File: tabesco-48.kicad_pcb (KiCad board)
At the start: 2 copper layers, 196.2 x 86.7 mm, 64 parts, among them U1 ProMicro

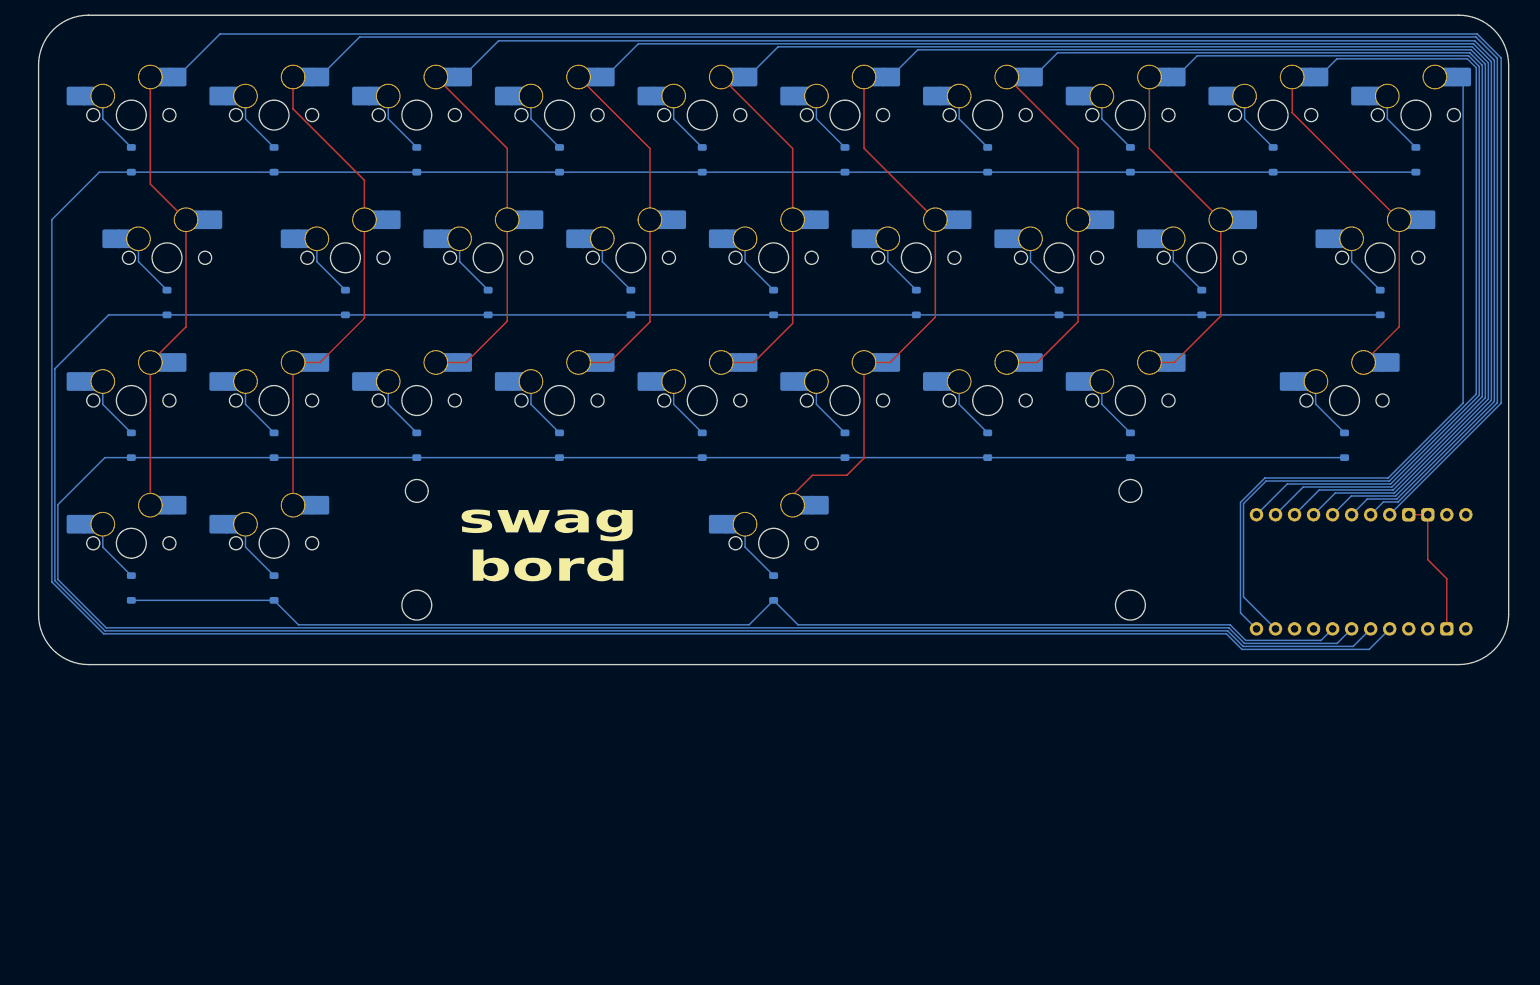
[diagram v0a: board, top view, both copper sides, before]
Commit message: more work, transitioning to IC in seperate repo
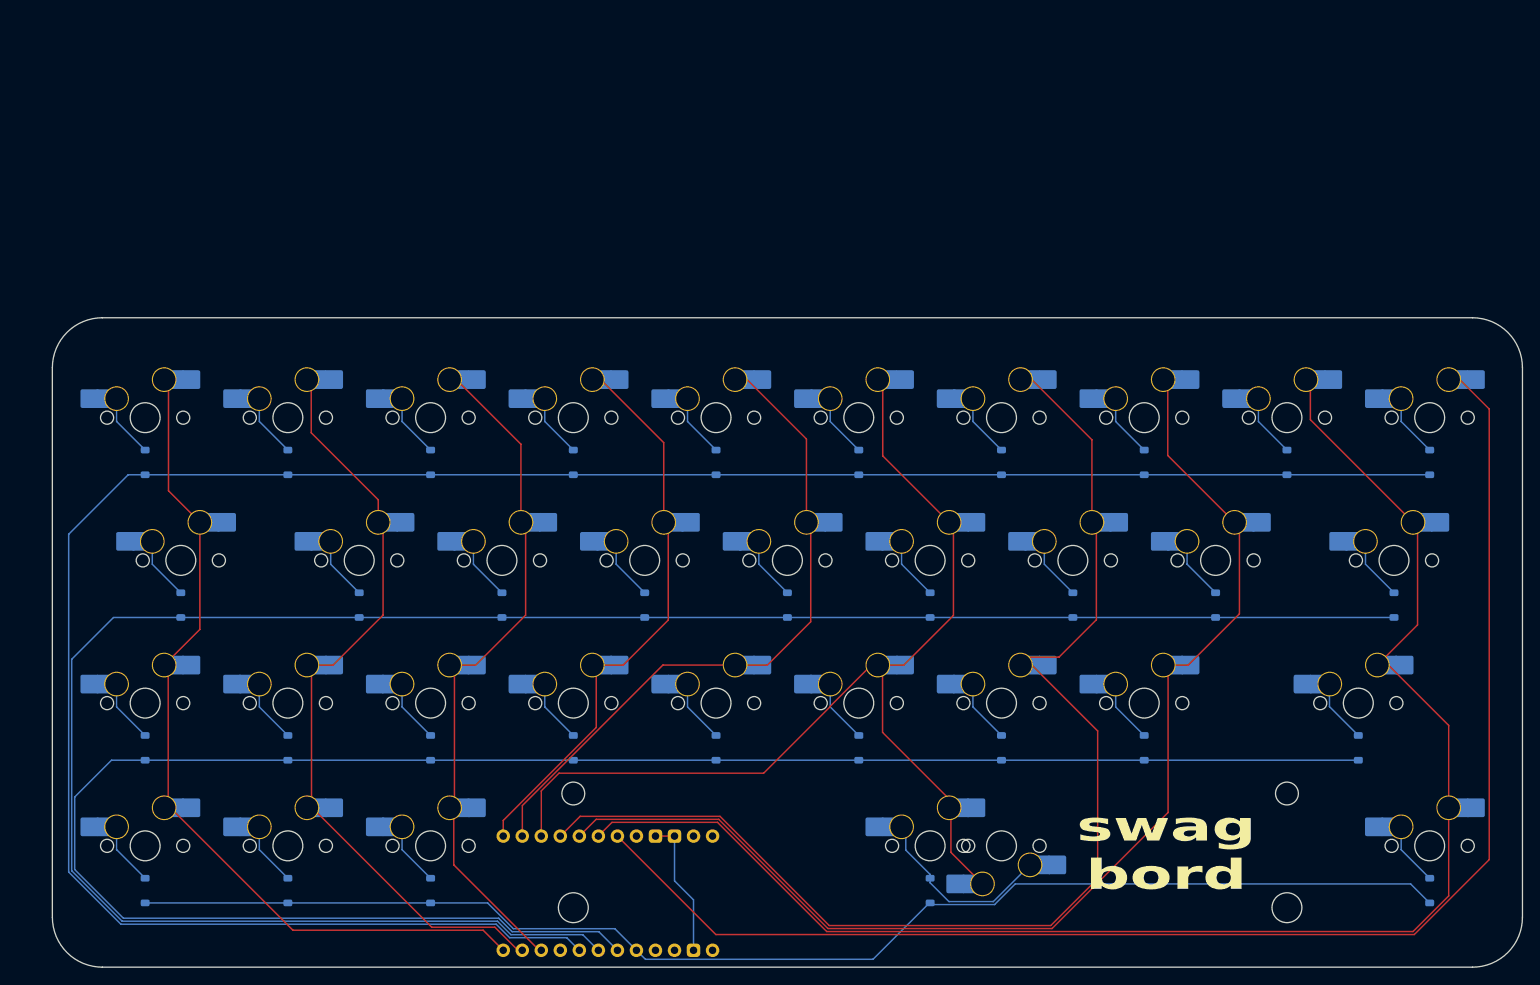
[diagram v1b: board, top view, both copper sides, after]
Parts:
- added D32: D_Small, Diode_SMD:D_SOD-123, B.Cu at (166.9, 135.7)
- added D34: D_Small, Diode_SMD:D_SOD-123, B.Cu at (233.6, 135.7)
- added MX32: MX_SW_HS, marbastlib-mx:SW_MX_HS_CPG151101S11_1u, B.Cu at (166.9, 129.7)
- added MX32-2: MX_SW_HS, marbastlib-mx:SW_MX_HS_CPG151101S11_1u, B.Cu at (176.4, 129.7)
- added MX34: MX_SW_HS, marbastlib-mx:SW_MX_HS_CPG151101S11_1u, B.Cu at (233.6, 129.7)
- moved U1 109.3 mm to (123.9, 136.1)
- moved D31 61.1 mm to (100.2, 135.7)
- moved MX31 61.1 mm to (100.2, 129.7)
- moved REF** 45.5 mm to (166.9, 129.7)
- moved D1 40.4 mm to (62.1, 78.6)
- moved D10 40.4 mm to (233.6, 78.6)
- moved D2 40.4 mm to (81.2, 78.6)
- moved D3 40.4 mm to (100.2, 78.6)
- moved D4 40.4 mm to (119.3, 78.6)
- moved D5 40.4 mm to (138.3, 78.6)
- moved D6 40.4 mm to (157.4, 78.6)
- moved D7 40.4 mm to (176.4, 78.6)
- moved D8 40.4 mm to (195.5, 78.6)
- moved D9 40.4 mm to (214.5, 78.6)
- moved D11 40.4 mm to (66.9, 97.6)
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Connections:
- MX31 pad 2: /col5 -> /col2
- U1 pad 11: /col6 -> /col4
- U1 pad 12: /col7 -> /col3
- U1 pad 17: /row0 -> /row3
- U1 pad 18: /row1 -> /row2
- U1 pad 19: /row2 -> /row1
- U1 pad 20: /row3 -> /row0
- U1 pad 22: unconnected-(U1-B3-Pad22) -> /col2
- U1 pad 23: /col8 -> /col1
- U1 pad 24: /col9 -> /col0
- U1 pad 5: /col0 -> unconnected-(U1-D1-Pad5)
- U1 pad 6: /col1 -> /col9
- U1 pad 7: /col2 -> /col8
- U1 pad 8: /col3 -> /col7
- U1 pad 9: /col4 -> /col6
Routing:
- net /col0: track 308.7 -> 114.7 mm
- net /col1: track 296.8 -> 104.8 mm
- net /col2: track 260.0 -> 92.9 mm
- net /col3: track 242.2 -> 77.8 mm
- net /col4: track 224.5 -> 90.2 mm
- net /row0: track 416.5 -> 302.5 mm
- net /row1: track 388.4 -> 281.7 mm
- net /row2: track 361.3 -> 259.9 mm
- net /col9: track 96.6 -> 193.1 mm
- net /col5: track 231.9 -> 141.4 mm
- net /col8: track 167.7 -> 204.4 mm
- net Net-(D32-A): track 0.00 -> 25.5 mm
- net /col6: track 188.7 -> 164.9 mm
- net /row3: track 165.9 -> 180.0 mm
- net /col7: track 171.2 -> 161.2 mm
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
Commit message: brain mode
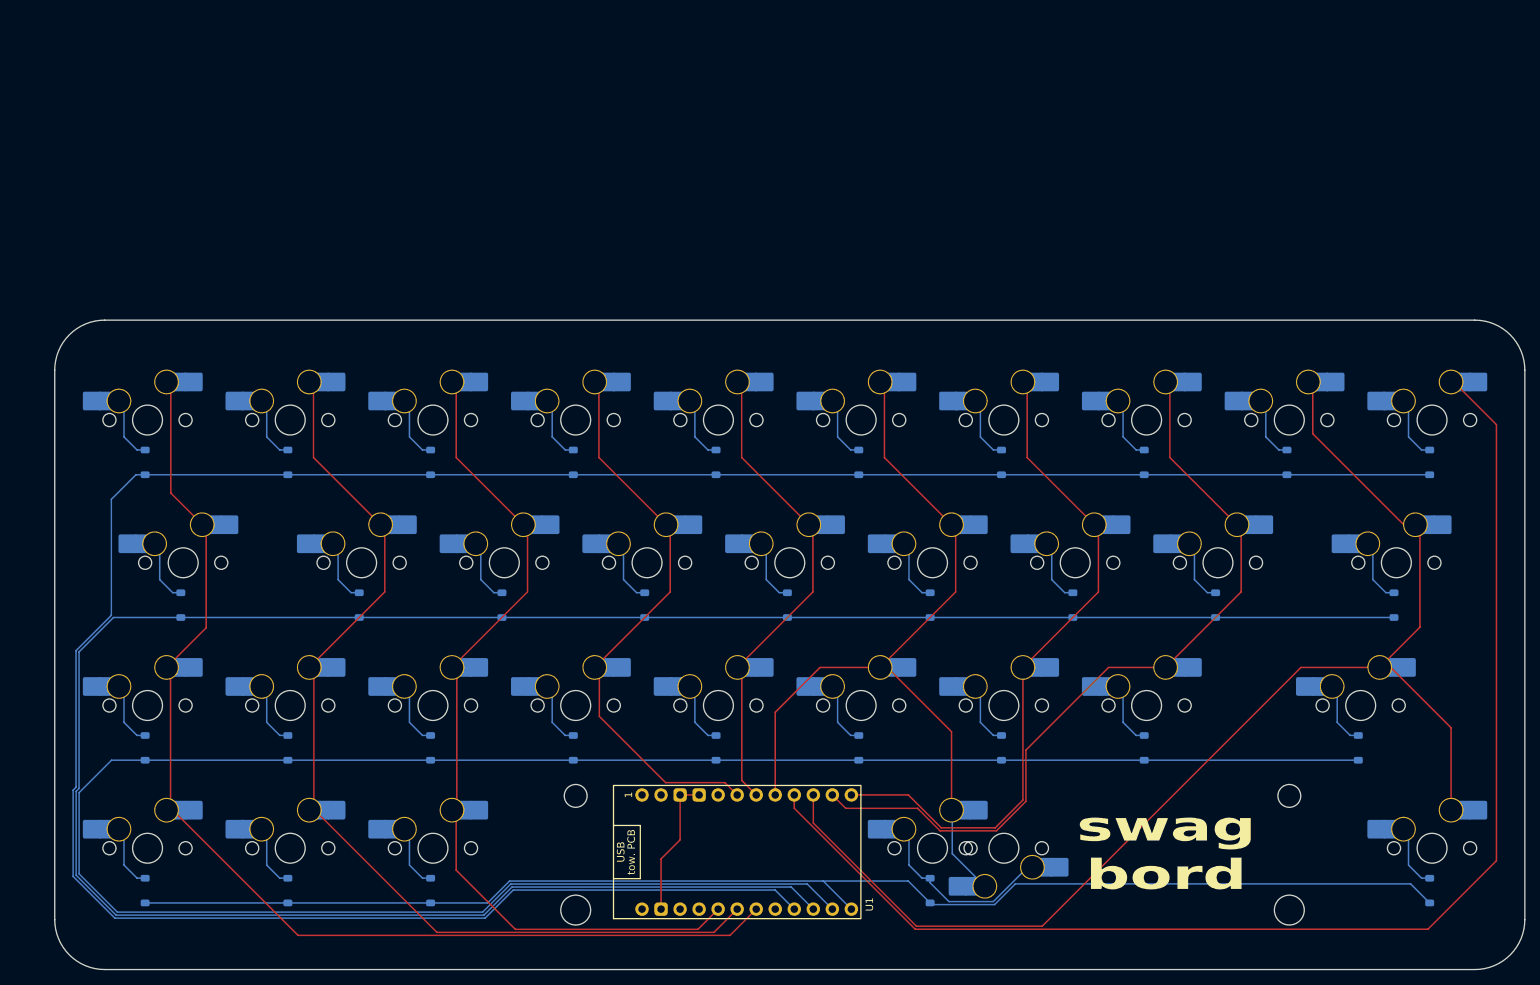
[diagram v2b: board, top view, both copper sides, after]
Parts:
- U1: moved to F.Cu
- moved U1 19.3 mm to (142.4, 130.6)
- moved MX7 0.45 mm to (176.7, 72.9)
- moved MX14 0.45 mm to (129.1, 91.9)
- moved MX26 0.45 mm to (176.7, 111.0)
- moved MX28 0.45 mm to (224.4, 111.0)
- moved MX32-2 0.45 mm to (176.7, 130.0)
- moved MX4 0.45 mm to (119.6, 72.9)
- moved MX1 0.45 mm to (62.4, 72.9)
- moved MX10 0.45 mm to (233.9, 72.9)
- moved MX11 0.45 mm to (67.2, 91.9)
- moved MX12 0.45 mm to (91.0, 91.9)
- moved MX2 0.45 mm to (81.5, 72.9)
- moved MX23 0.45 mm to (119.6, 111.0)
- moved MX3 0.45 mm to (100.5, 72.9)
- moved MX5 0.45 mm to (138.6, 72.9)
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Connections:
- U1 pad 10: /col5 -> /col8
- U1 pad 11: /col4 -> /col7
- U1 pad 12: /col3 -> /col6
- U1 pad 17: /row3 -> /col2
- U1 pad 18: /row2 -> /col1
- U1 pad 19: /row1 -> /col0
- U1 pad 20: /row0 -> unconnected-(U1-F7-Pad20)
- U1 pad 21: unconnected-(U1-B1-Pad21) -> /row0
- U1 pad 22: /col2 -> /row1
- U1 pad 23: /col1 -> /row2
- U1 pad 24: /col0 -> /row3
- U1 pad 6: /col9 -> /col3
- U1 pad 7: /col8 -> /col4
- U1 pad 8: /col7 -> /col5
- U1 pad 9: /col6 -> /col9
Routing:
- net /col6: track 164.9 -> 91.9 mm
- net /col7: track 161.2 -> 107.6 mm
- net /col0: track 114.7 -> 149.0 mm
- net /col8: track 204.4 -> 170.6 mm
- net /col5: track 141.4 -> 110.8 mm
- net /row2: track 259.9 -> 288.5 mm
- net /row1: track 281.7 -> 310.3 mm
- net /row0: track 302.5 -> 330.5 mm
- net /col1: track 104.8 -> 131.2 mm
- net /col4: track 90.2 -> 64.5 mm
- net /col2: track 92.9 -> 113.6 mm
- net /col9: track 193.1 -> 174.1 mm
- net /row3: track 180.0 -> 181.6 mm
- net /col3: track 77.8 -> 76.7 mm

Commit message: finished tabesco-34
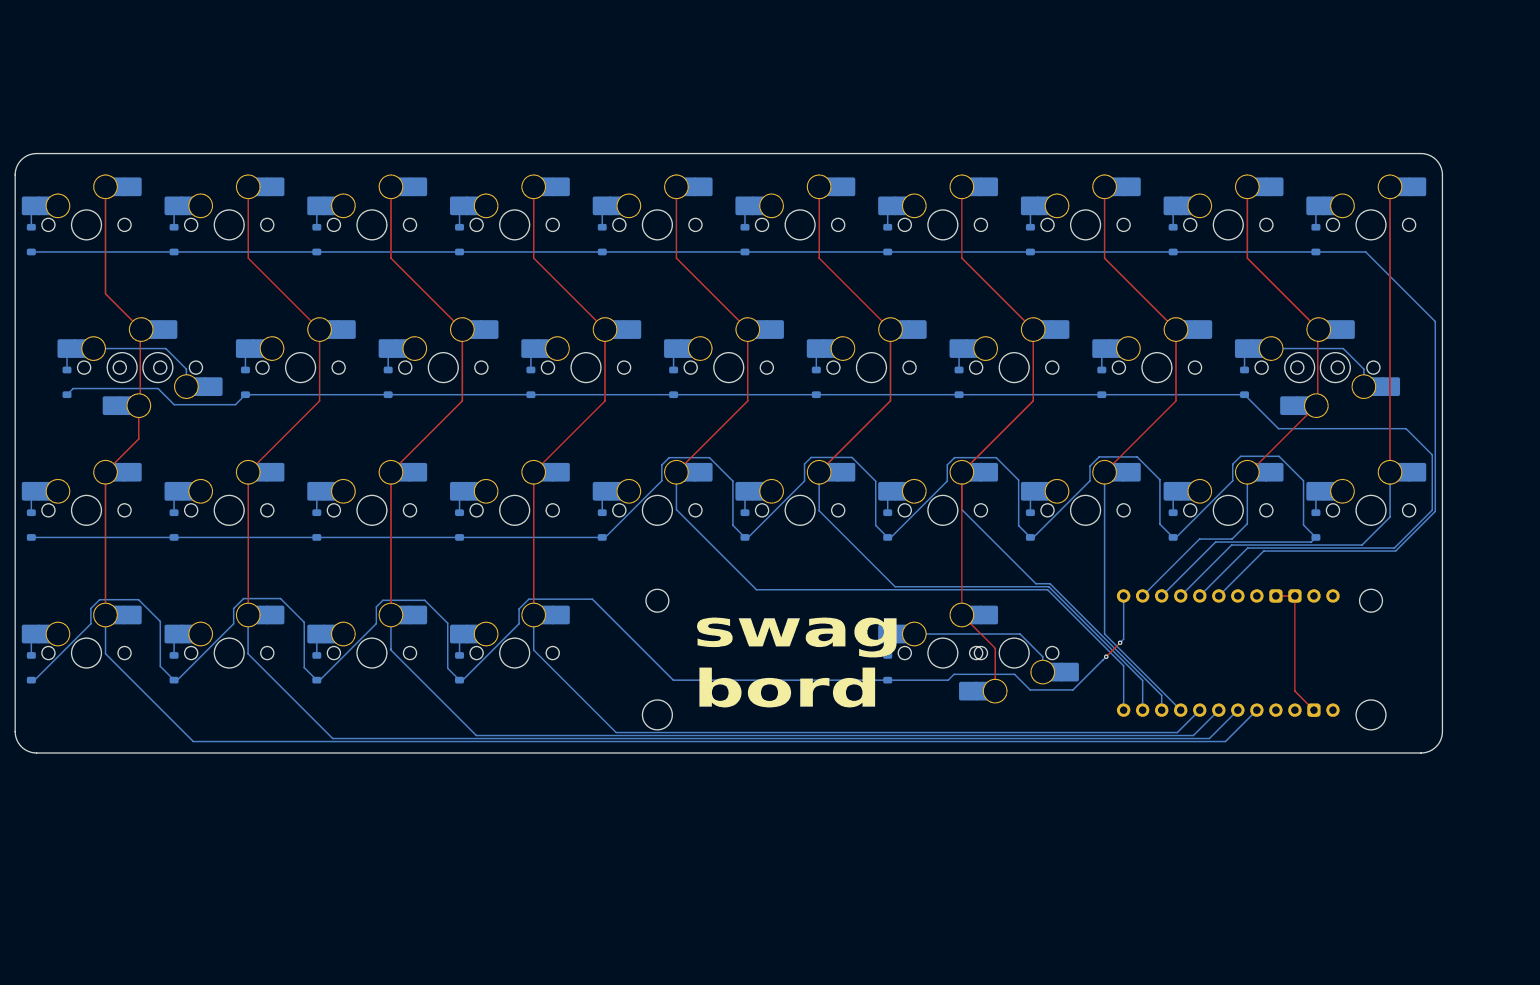
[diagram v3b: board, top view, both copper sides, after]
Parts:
- removed MX32-2: MX_SW_HS, marbastlib-mx:SW_MX_HS_CPG151101S11_1u
- added D33: D_Small, Diode_SMD:D_SOD-123, B.Cu at (104.1, 106.0)
- added MX11-2: MX_SW_HS, marbastlib-mx:SW_MX_HS_CPG151101S11_1u, B.Cu at (63.8, 65.9)
- added MX19-2: MX_SW_HS, marbastlib-mx:SW_MX_HS_CPG151101S11_1u, B.Cu at (221.0, 65.9)
- added MX33: MX_SW_HS, marbastlib-mx:SW_MX_HS_CPG151101S11_1u, B.Cu at (111.4, 104.0)
- added MX34-2: MX_SW_HS, marbastlib-mx:SW_MX_HS_CPG151101S11_1u, B.Cu at (178.1, 104.0)
- U1: moved to B.Cu
- moved MX29 169.4 mm to (225.7, 84.9)
- moved D29 163.7 mm to (218.4, 86.9)
- moved D32 87.1 mm to (85.0, 106.0)
- moved MX32 79.2 mm to (92.4, 104.0)
- moved D34 78.2 mm to (161.2, 106.0)
- moved MX34 70.3 mm to (168.6, 104.0)
- moved U1 69.6 mm to (206.7, 104.0)
- moved D30 45.3 mm to (46.9, 106.0)
- moved D31 45.3 mm to (66.0, 106.0)
- moved D28 38.7 mm to (199.3, 86.9)
- moved MX30 37.7 mm to (54.3, 104.0)
- moved MX31 37.7 mm to (73.3, 104.0)
- moved D19 35.8 mm to (208.9, 67.9)
- moved D1 33.4 mm to (46.9, 48.8)
- moved D10 33.4 mm to (218.4, 48.8)
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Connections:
- D29 pad 1: /row3 -> /row2
- MX29 pad 2: /col0 -> /col9
- MX30 pad 2: /col1 -> /col0
- MX31 pad 2: /col2 -> /col1
- MX32 pad 2: /col5 -> /col2
- MX34 pad 2: /col8 -> /col6
- U1 pad 10: /col8 -> /row2
- U1 pad 11: /col7 -> /col8
- U1 pad 12: /col6 -> /row3
- U1 pad 17: /col2 -> /col0
- U1 pad 19: /col0 -> /col2
- U1 pad 20: unconnected-(U1-F7-Pad20) -> /col3
- U1 pad 21: /row0 -> /col7
- U1 pad 22: /row1 -> /col6
- U1 pad 23: /row2 -> /col5
- U1 pad 24: /row3 -> /col4
- U1 pad 6: /col3 -> unconnected-(U1-D0-Pad6)
- U1 pad 7: /col4 -> /row0
- U1 pad 8: /col5 -> /row1
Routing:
- net /col8: track 170.6 -> 71.0 mm
- net /col9: track 174.1 -> 76.4 mm
- net /col3: track 76.7 -> 164.4 mm
- net /row0: track 330.5 -> 250.1 mm
- net /row1: track 310.3 -> 230.5 mm
- net /col0: track 149.0 -> 226.5 mm
- net /col1: track 131.2 -> 208.6 mm
- net /col2: track 113.6 -> 186.4 mm
- net /col4: track 64.5 -> 125.2 mm
- net /col6: track 91.9 -> 120.9 mm
- net /col7: track 107.6 -> 81.9 mm
- net /row2: track 288.5 -> 263.3 mm
- net /row3: track 181.6 -> 206.7 mm, vias 0 -> 2
- net Net-(D32-A): track 25.6 -> 2.86 mm
- net Net-(D34-A): track 8.63 -> 23.3 mm
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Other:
- board size 196.2 x 86.7 mm -> 190.5 x 80 mm
- board text added: "tabesco-34"
- board text removed: "tabesco-31"
